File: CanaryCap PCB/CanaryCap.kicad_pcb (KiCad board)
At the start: 2 copper layers, 120 x 30 mm, 59 parts, among them J1 USB_C_Receptacle_USB2.0_16P, J2 Impact Connector, J3 Gas Connector, J4 Battery Connector, Q1 NMOS, Q2 PMOS_Substrate, SW1 SW_MEC_5E, SW2 SW_MEC_5E, SW3 SW_MEC_5E, U1 LMZM23601V5, U2 LM3940 3.3V-SOT223, U3 ESP32-C6FH4, U4 ADXL343

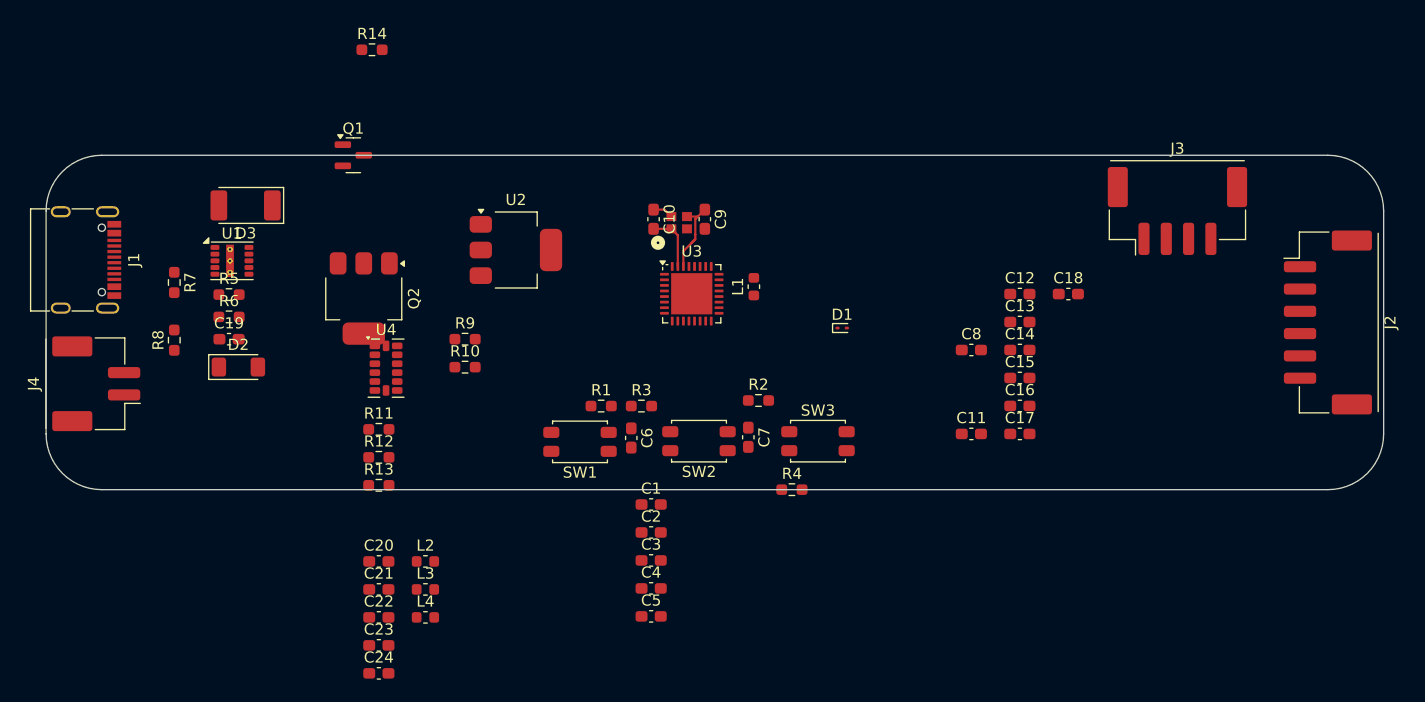
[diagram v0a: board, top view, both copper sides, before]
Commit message: FIXED IT MF
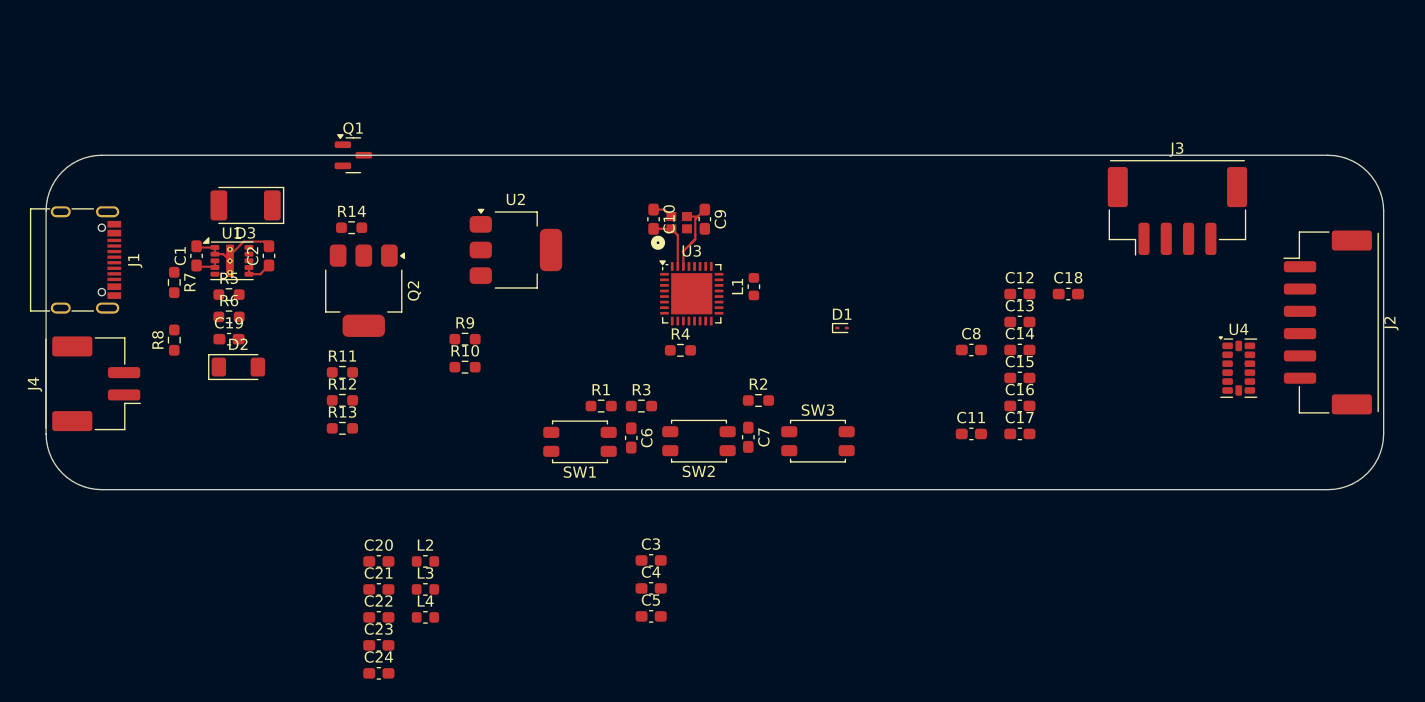
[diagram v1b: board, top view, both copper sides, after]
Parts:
- moved U4 76.5 mm to (207.5, -10.9)
- moved C1 46.5 mm to (114.0, -21.0), turned to 90 degrees
- moved C2 42.3 mm to (120.5, -21.0), turned to 90 degrees
- moved R14 16.1 mm to (127.9, -23.5)
- moved R4 16.0 mm to (157.4, -12.5)
- moved R11 6.06 mm to (127.1, -10.5)
- moved R12 6.06 mm to (127.1, -8.01)
- moved R13 6.06 mm to (127.1, -5.50)
- moved Q2 0.70 mm to (129.0, -17.9)
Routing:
- net GNDREF: track 1.86 -> 10.4 mm
- net +5V_buck: track 0.00 -> 2.72 mm
- net +12V: track 0.00 -> 2.28 mm
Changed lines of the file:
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@@
 	(footprint "Resistor_SMD:R_0603_1608Metric_Pad0.98x0.95mm_HandSolder"
 		(layer "F.Cu")
-		(at 130.353301 -0.389701)
+		(at 127.0875 -5.5)
 		(descr "Resistor SMD 0603 (1608 Metric), square (rectangular) end terminal, IPC-7351 nominal with elongated pad for handsoldering. (Body size source: IPC-SM-782 page 72, https://www.pcb-3d.com/wordpress/wp-content/uploads/ipc-sm-782a_amendment_1_and_2.pdf), generated with kicad-footprint-generator")
 		(tags "resistor handsolder")
@@
 	(footprint "Resistor_SMD:R_0603_1608Metric_Pad0.98x0.95mm_HandSolder"
 		(layer "F.Cu")
-		(at 130.353301 -2.899701)
+		(at 127.0875 -8.01)
 		(descr "Resistor SMD 0603 (1608 Metric), square (rectangular) end terminal, IPC-7351 nominal with elongated pad for handsoldering. (Body size source: IPC-SM-782 page 72, https://www.pcb-3d.com/wordpress/wp-content/uploads/ipc-sm-782a_amendment_1_and_2.pdf), generated with kicad-footprint-generator")
 		(tags "resistor handsolder")
@@
 	(footprint "Resistor_SMD:R_0603_1608Metric_Pad0.98x0.95mm_HandSolder"
 		(layer "F.Cu")
-		(at 130.353301 -5.409701)
+		(at 127.0875 -10.52)
 		(descr "Resistor SMD 0603 (1608 Metric), square (rectangular) end terminal, IPC-7351 nominal with elongated pad for handsoldering. (Body size source: IPC-SM-782 page 72, https://www.pcb-3d.com/wordpress/wp-content/uploads/ipc-sm-782a_amendment_1_and_2.pdf), generated with kicad-footprint-generator")
 		(tags "resistor handsolder")
@@
 	(footprint "Capacitor_SMD:C_0603_1608Metric_Pad1.08x0.95mm_HandSolder"
 		(layer "F.Cu")
-		(at 154.783301 3.840299)
+		(at 120.5 -20.975 90)
 		(descr "Capacitor SMD 0603 (1608 Metric), square (rectangular) end terminal, IPC-7351 nominal with elongated pad for handsoldering. (Body size source: IPC-SM-782 page 76, https://www.pcb-3d.com/wordpress/wp-content/uploads/ipc-sm-782a_amendment_1_and_2.pdf), generated with kicad-footprint-generator")
 		(tags "capacitor handsolder")
 		(property "Reference" "C2"
-			(at 0 -1.43 0)
+			(at 0 -1.43 90)
 			(layer "F.SilkS")
 			(effects
@@
 		)
 		(property "Value" "10uF"
-			(at 0 1.43 0)
+			(at 0 1.43 90)
 			(layer "F.Fab")
 			(effects
@@
 		)
 		(property "Datasheet" "~"
-			(at 0 0 0)
+			(at 0 0 90)
 			(layer "F.Fab")
 			(hide yes)
@@
 		)
 		(property "Description" "Unpolarized capacitor"
-			(at 0 0 0)
+			(at 0 0 90)
 			(layer "F.Fab")
 			(hide yes)
@@
 		)
 		(fp_line
-			(start -1.65 -0.73)
-			(end 1.65 -0.73)
+			(start 1.65 -0.73)
+			(end 1.65 0.73)
 			(stroke
 				(width 0.05)
@@
 		)
 		(fp_line
-			(start -1.65 0.73)
-			(end -1.65 -0.73)
+			(start -1.65 -0.73)
+			(end 1.65 -0.73)
 			(stroke
 				(width 0.05)
@@
 		)
 		(fp_line
-			(start 1.65 -0.73)
-			(end 1.65 0.73)
+			(start 1.65 0.73)
+			(end -1.65 0.73)
 			(stroke
 				(width 0.05)
@@
 		)
 		(fp_line
-			(start 1.65 0.73)
-			(end -1.65 0.73)
+			(start -1.65 0.73)
+			(end -1.65 -0.73)
 			(stroke
 				(width 0.05)
@@
 		)
 		(fp_line
-			(start -0.8 -0.4)
-			(end 0.8 -0.4)
+			(start 0.8 -0.4)
+			(end 0.8 0.4)
 			(stroke
 				(width 0.1)
@@
 		)
 		(fp_line
-			(start -0.8 0.4)
-			(end -0.8 -0.4)
+			(start -0.8 -0.4)
+			(end 0.8 -0.4)
 			(stroke
 				(width 0.1)
@@
 		)
 		(fp_line
-			(start 0.8 -0.4)
-			(end 0.8 0.4)
+			(start 0.8 0.4)
+			(end -0.8 0.4)
 			(stroke
 				(width 0.1)
@@
 		)
 		(fp_line
-			(start 0.8 0.4)
-			(end -0.8 0.4)
+			(start -0.8 0.4)
+			(end -0.8 -0.4)
 			(stroke
 				(width 0.1)
@@
 		)
 		(fp_text user "${REFERENCE}"
-			(at 0 0 0)
+			(at 0 0 90)
 			(layer "F.Fab")
 			(effects
@@
 		)
 		(pad "1" smd roundrect
-			(at -0.8625 0)
+			(at -0.8625 0 90)
 			(size 1.075 0.95)
 			(layers "F.Cu" "F.Mask" "F.Paste")
@@
 		)
 		(pad "2" smd roundrect
-			(at 0.8625 0)
+			(at 0.8625 0 90)
 			(size 1.075 0.95)
 			(layers "F.Cu" "F.Mask" "F.Paste")
@@
 	(footprint "Package_TO_SOT_SMD:SOT-223"
 		(layer "F.Cu")
-		(at 129 -17.15 -90)
+		(at 129 -17.85 -90)
 		(descr "module CMS SOT223 4 pins")
 		(tags "CMS SOT")
@@
 	(footprint "Resistor_SMD:R_0603_1608Metric_Pad0.98x0.95mm_HandSolder"
 		(layer "F.Cu")
-		(at 129.7425 -39.465)
+		(at 127.9125 -23.5)
 		(descr "Resistor SMD 0603 (1608 Metric), square (rectangular) end terminal, IPC-7351 nominal with elongated pad for handsoldering. (Body size source: IPC-SM-782 page 72, https://www.pcb-3d.com/wordpress/wp-content/uploads/ipc-sm-782a_amendment_1_and_2.pdf), generated with kicad-footprint-generator")
 		(tags "resistor handsolder")
@@
 		)
 		(property "Value" "0OHM if needed"
-			(at 0 1.43 0)
+			(at 0.0875 -1.5 0)
 			(layer "F.Fab")
 			(effects
@@
 	(footprint "Resistor_SMD:R_0603_1608Metric_Pad0.98x0.95mm_HandSolder"
 		(layer "F.Cu")
-		(at 167.4125 0)
+		(at 157.4125 -12.5)
 		(descr "Resistor SMD 0603 (1608 Metric), square (rectangular) end terminal, IPC-7351 nominal with elongated pad for handsoldering. (Body size source: IPC-SM-782 page 72, https://www.pcb-3d.com/wordpress/wp-content/uploads/ipc-sm-782a_amendment_1_and_2.pdf), generated with kicad-footprint-generator")
 		(tags "resistor handsolder")
@@
 	(footprint "Package_LGA:LGA-14_3x5mm_P0.8mm_LayoutBorder1x6y"
 		(layer "F.Cu")
-		(at 131 -10.9)
+		(at 207.5 -10.9)
 		(descr "LGA, 14 Pin (http://www.st.com/resource/en/datasheet/lsm303dlhc.pdf), generated with kicad-footprint-generator ipc_noLead_generator.py")
 		(tags "LGA NoLead")
@@
 	(footprint "Capacitor_SMD:C_0603_1608Metric_Pad1.08x0.95mm_HandSolder"
 		(layer "F.Cu")
-		(at 154.783301 1.330299)
+		(at 114 -20.975 90)
 		(descr "Capacitor SMD 0603 (1608 Metric), square (rectangular) end terminal, IPC-7351 nominal with elongated pad for handsoldering. (Body size source: IPC-SM-782 page 76, https://www.pcb-3d.com/wordpress/wp-content/uploads/ipc-sm-782a_amendment_1_and_2.pdf), generated with kicad-footprint-generator")
 		(tags "capacitor handsolder")
 		(property "Reference" "C1"
-			(at 0 -1.43 0)
+			(at 0 -1.43 90)
 			(layer "F.SilkS")
 			(effects
@@
 		)
 		(property "Value" "10uF"
-			(at 0 1.43 0)
+			(at 0 1.43 90)
 			(layer "F.Fab")
 			(effects
@@
 		)
 		(property "Datasheet" "~"
-			(at 0 0 0)
+			(at 0 0 90)
 			(layer "F.Fab")
 			(hide yes)
@@
 		)
 		(property "Description" "Unpolarized capacitor"
-			(at 0 0 0)
+			(at 0 0 90)
 			(layer "F.Fab")
 			(hide yes)
@@
 		)
 		(fp_line
-			(start -1.65 -0.73)
-			(end 1.65 -0.73)
+			(start 1.65 -0.73)
+			(end 1.65 0.73)
 			(stroke
 				(width 0.05)
@@
 		)
 		(fp_line
-			(start -1.65 0.73)
-			(end -1.65 -0.73)
+			(start -1.65 -0.73)
+			(end 1.65 -0.73)
 			(stroke
 				(width 0.05)
@@
 		)
 		(fp_line
-			(start 1.65 -0.73)
-			(end 1.65 0.73)
+			(start 1.65 0.73)
+			(end -1.65 0.73)
 			(stroke
 				(width 0.05)
@@
 		)
 		(fp_line
-			(start 1.65 0.73)
-			(end -1.65 0.73)
+			(start -1.65 0.73)
+			(end -1.65 -0.73)
 			(stroke
 				(width 0.05)
@@
 		)
 		(fp_line
-			(start -0.8 -0.4)
-			(end 0.8 -0.4)
+			(start 0.8 -0.4)
+			(end 0.8 0.4)
 			(stroke
 				(width 0.1)
@@
 		)
 		(fp_line
-			(start -0.8 0.4)
-			(end -0.8 -0.4)
+			(start -0.8 -0.4)
+			(end 0.8 -0.4)
 			(stroke
 				(width 0.1)
@@
 		)
 		(fp_line
-			(start 0.8 -0.4)
-			(end 0.8 0.4)
+			(start 0.8 0.4)
+			(end -0.8 0.4)
 			(stroke
 				(width 0.1)
@@
 		)
 		(fp_line
-			(start 0.8 0.4)
-			(end -0.8 0.4)
+			(start -0.8 0.4)
+			(end -0.8 -0.4)
 			(stroke
 				(width 0.1)
@@
 		)
 		(fp_text user "${REFERENCE}"
-			(at 0 0 0)
+			(at 0 0 90)
 			(layer "F.Fab")
 			(effects
@@
 		)
 		(pad "1" smd roundrect
-			(at -0.8625 0)
+			(at -0.8625 0 90)
 			(size 1.075 0.95)
 			(layers "F.Cu" "F.Mask" "F.Paste")
@@
 		)
 		(pad "2" smd roundrect
-			(at 0.8625 0)
+			(at 0.8625 0 90)
 			(size 1.075 0.95)
 			(layers "F.Cu" "F.Mask" "F.Paste")
@@
 	)
 	(segment
+		(start 115.65 -21.13)
+		(end 115.65 -21.73)
+		(width 0.2)
+		(layer "F.Cu")
+		(net 1)
+	)
+	(segment
+		(start 118.238106 -22.256)
+		(end 120.0815 -22.256)
+		(width 0.2)
+		(layer "F.Cu")
+		(net 1)
+	)
+	(segment
+		(start 120.0815 -22.256)
+		(end 120.5 -21.8375)
+		(width 0.2)
+		(layer "F.Cu")
+		(net 1)
+	)
+	(segment
 		(start 155 -25.125002)
 		(end 155.974996 -25.125002)
@@
 	)
 	(segment
+		(start 117 -21.017894)
+		(end 118.238106 -22.256)
+		(width 0.2)
+		(layer "F.Cu")
+		(net 1)
+	)
+	(segment
+		(start 114 -21.725)
+		(end 115.645 -21.725)
+		(width 0.2)
+		(layer "F.Cu")
+		(net 1)
+	)
+	(segment
+		(start 117 -20.53)
+		(end 117 -21.017894)
+		(width 0.2)
+		(layer "F.Cu")
+		(net 1)
+	)
+	(segment
+		(start 115.645 -21.725)
+		(end 115.65 -21.73)
+		(width 0.2)
+		(layer "F.Cu")
+		(net 1)
+	)
+	(segment
+		(start 116.4 -21.13)
+		(end 117 -20.53)
+		(width 0.2)
+		(layer "F.Cu")
+		(net 1)
+	)
+	(segment
 		(start 155.974996 -25.125002)
 		(end 156.599998 -24.5)
@@
 	)
 	(segment
+		(start 115.65 -21.13)
+		(end 116.4 -21.13)
+		(width 0.2)
+		(layer "F.Cu")
+		(net 1)
+	)
+	(segment
+		(start 115.58 -20)
+		(end 115.65 -19.93)
+		(width 0.2)
+		(layer "F.Cu")
+		(net 2)
+	)
+	(segment
+		(start 115.65 -19.93)
+		(end 115.65 -20.53)
+		(width 0.2)
+		(layer "F.Cu")
+		(net 2)
+	)
+	(segment
+		(start 114 -20)
+		(end 115.58 -20)
+		(width 0.2)
+		(layer "F.Cu")
+		(net 2)
+	)
+	(segment
+		(start 119.7175 -19.33)
+		(end 120.5 -20.1125)
+		(width 0.2)
+		(layer "F.Cu")
+		(net 3)
+	)
+	(segment
+		(start 118.7 -19.33)
+		(end 119.7175 -19.33)
+		(width 0.2)
+		(layer "F.Cu")
+		(net 3)
+	)
+	(segment
+		(start 118.7 -19.33)
+		(end 118.7 -19.93)
+		(width 0.2)
+		(layer "F.Cu")
+		(net 3)
+	)
+	(segment
